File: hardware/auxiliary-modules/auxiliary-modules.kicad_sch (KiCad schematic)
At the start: 38 parts, among them J1 IDC-10, J2 Conn_01x07, J3 Conn_01x04, J4 IDC-10, J5 IDC-10, U1 CS49E, U2 NTS0102, U3 LM393, U4 NTS0102

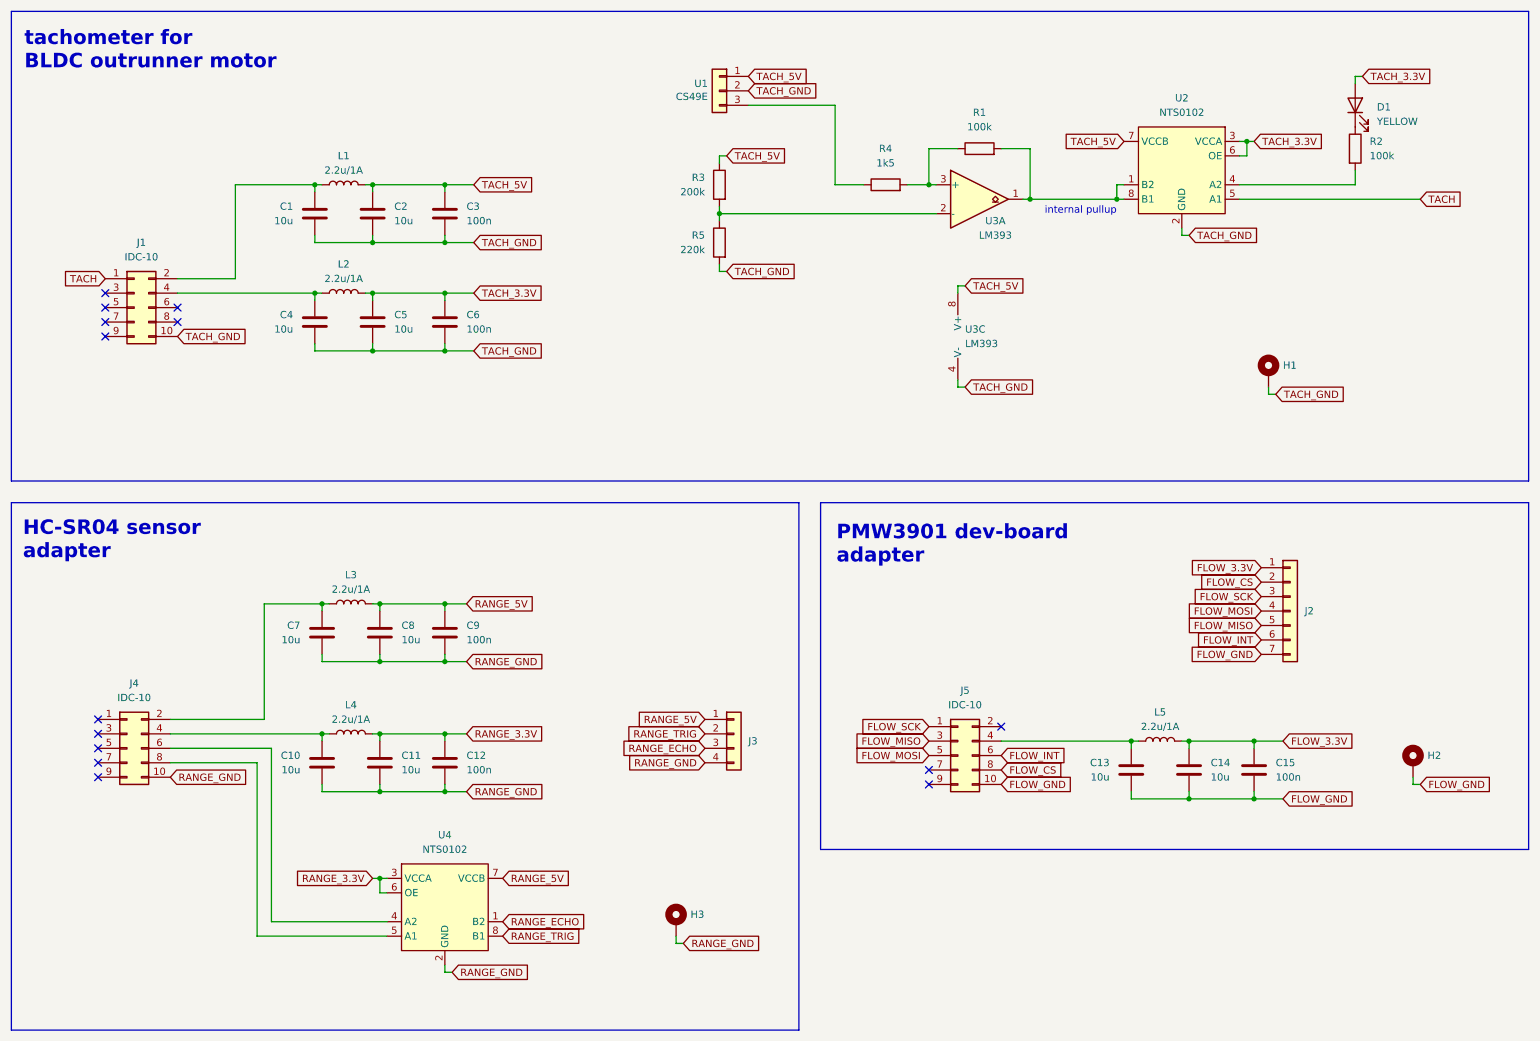
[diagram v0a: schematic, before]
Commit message: Mouser
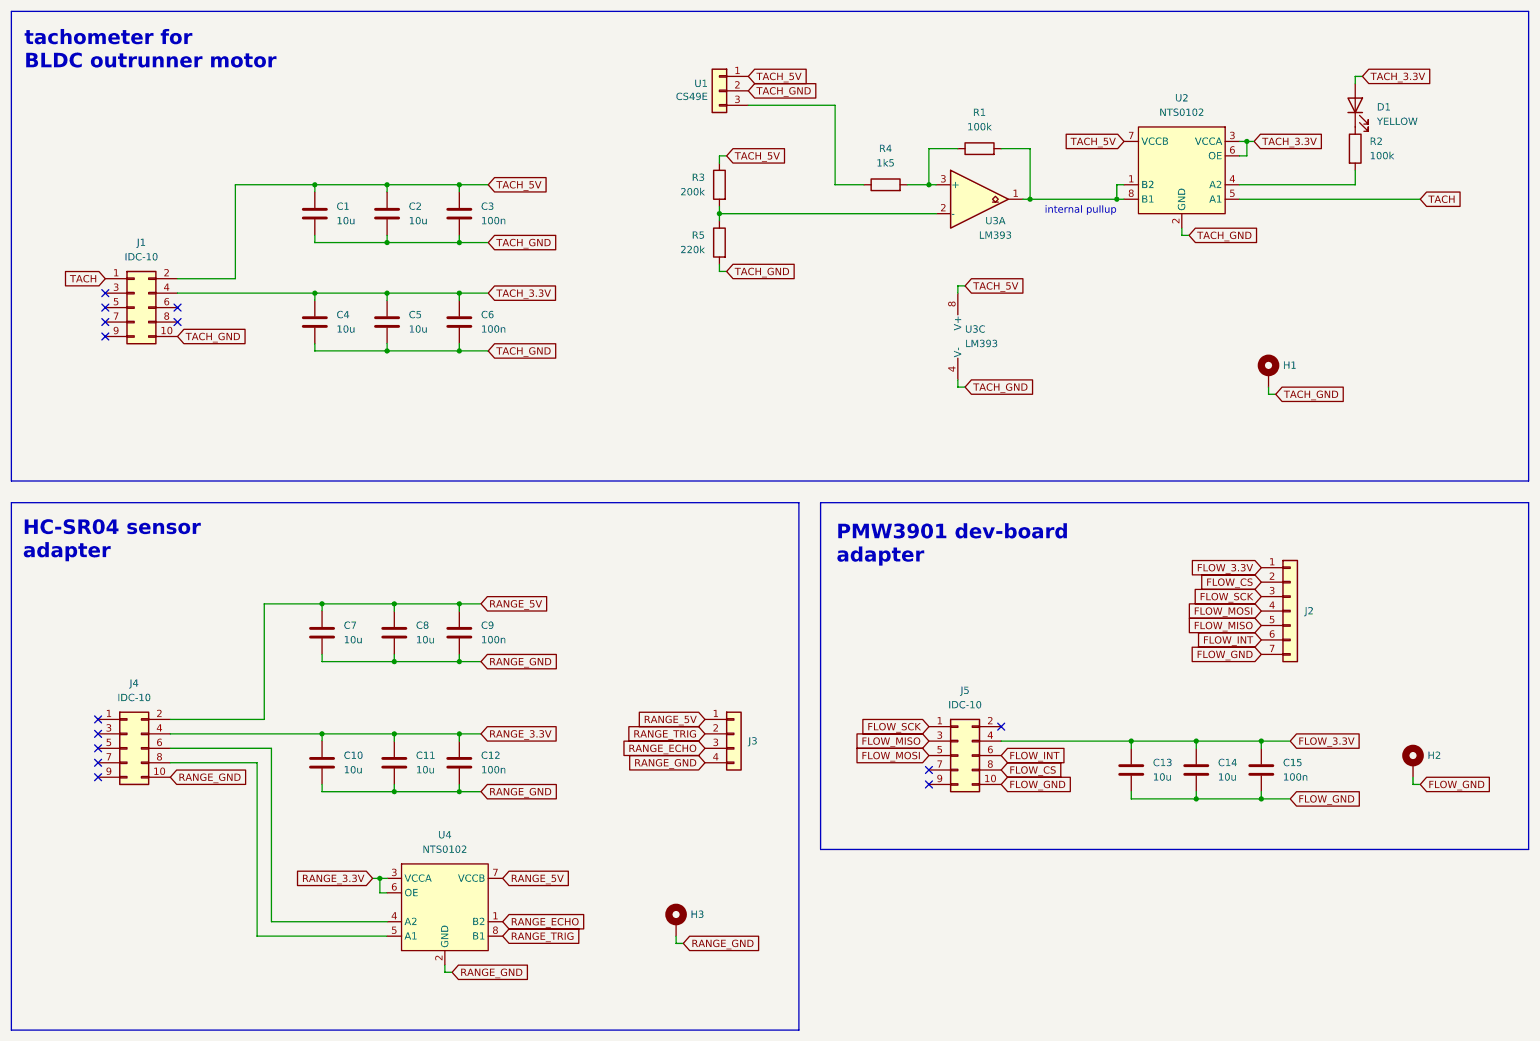
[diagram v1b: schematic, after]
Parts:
- removed L1, L2, L3, L4, L5: 2.2u/1A, Inductor_SMD:L_0603_1608Metric, symbol Device:L
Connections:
- net FLOW_3.3V: now also C13.1, J5.4 (Pin_4)
- net RANGE_3.3V: now also C10.1, J4.4 (Pin_4)
- net RANGE_5V: now also C7.1, J4.2 (Pin_2)
- net TACH_3.3V: now also C4.1, J1.4 (Pin_4)
- net TACH_5V: now also C1.1, J1.2 (Pin_2)
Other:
- moved on the sheet: C11, C12, C14, C15, C2, C3, C5, C6, C8, C9
